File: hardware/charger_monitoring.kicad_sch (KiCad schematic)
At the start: 24 parts, among them Q2801 IRFR120NTRPBF, Q2802 IPT015N10N5, Q2803 IPT015N10N5, U2802 BQ76200PW, U4 ACS770xCB-050B-PFF

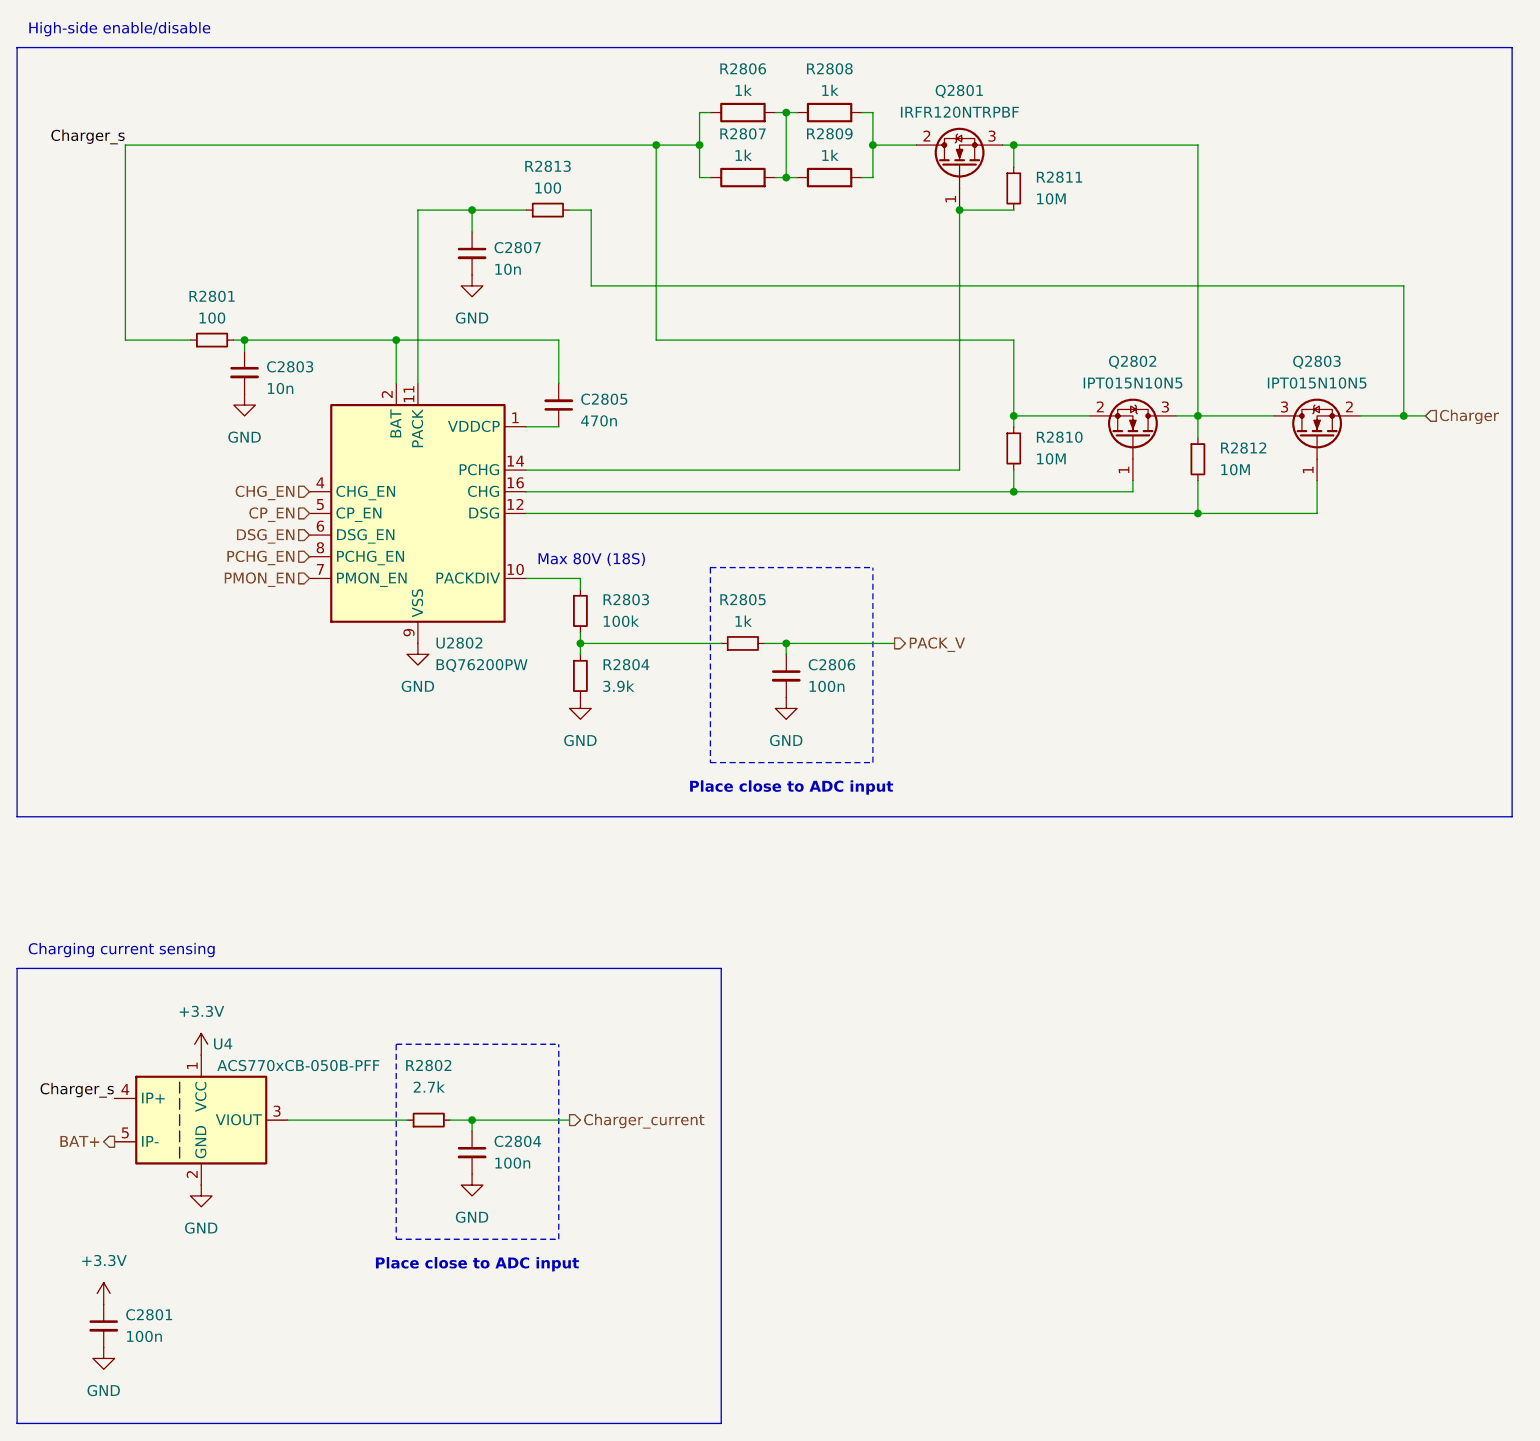
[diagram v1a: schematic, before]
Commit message: Fix OLED pinout and add HDC1080
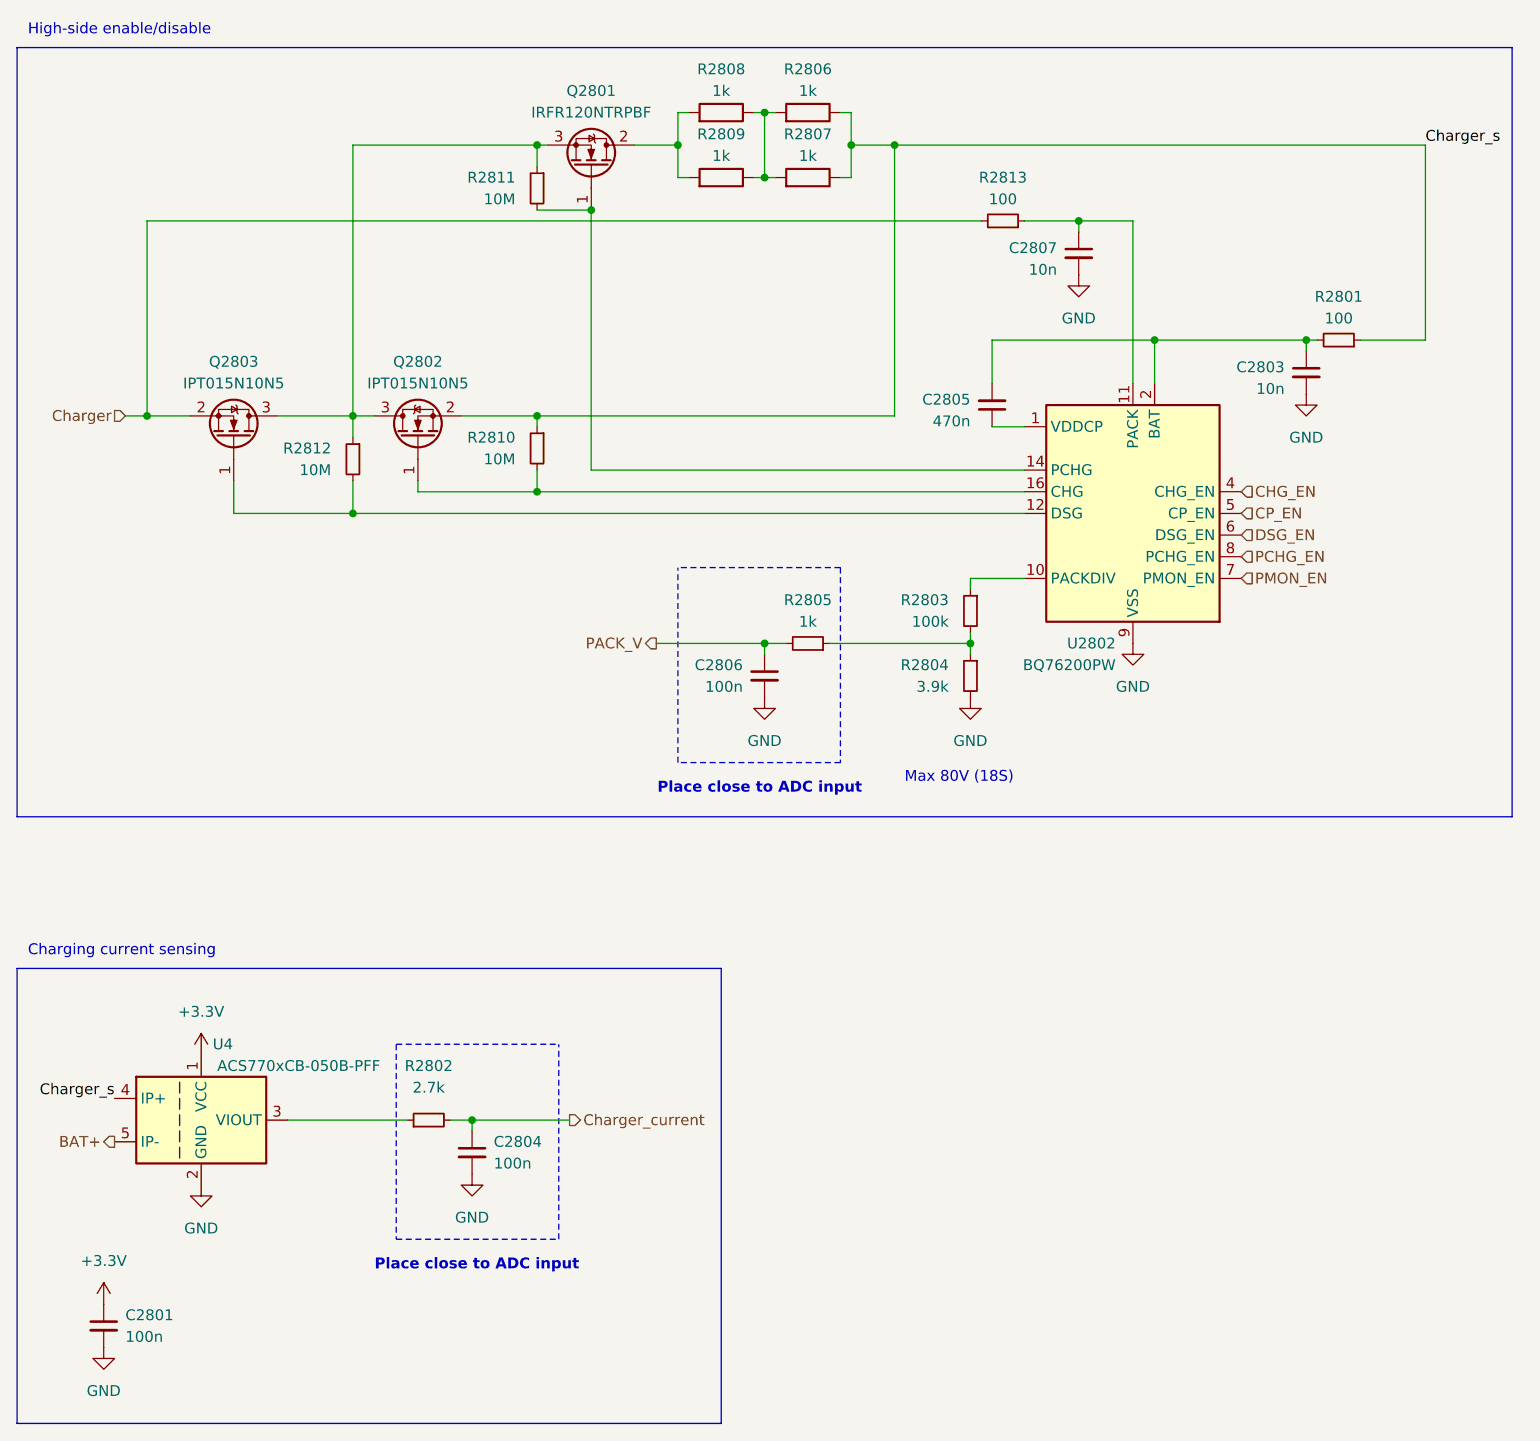
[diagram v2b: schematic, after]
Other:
- moved on the sheet: C2803, C2805, C2806, C2807, Q2801, Q2802, Q2803, R2801, R2803, R2804, R2805, R2806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
